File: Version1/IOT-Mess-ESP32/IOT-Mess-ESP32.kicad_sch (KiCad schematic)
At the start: 26 parts, among them J1 Conn_01x19_Pin, J10 Jumper, J2 Conn_01x19_Pin, J3 Jumper_2, J4 Jumper_2, J5 Conn_01x06_Pin, J7 Jumper, J8 Jumper, J9 Jumper, SW10 SW_Push, SW11 SW_Push, U10 USB_C_Receptacle_USB2.0_16P, U2 ESP32-C6-MINI-1, U4 ESP32-S2-WROVER, U6 ME6211C33M5

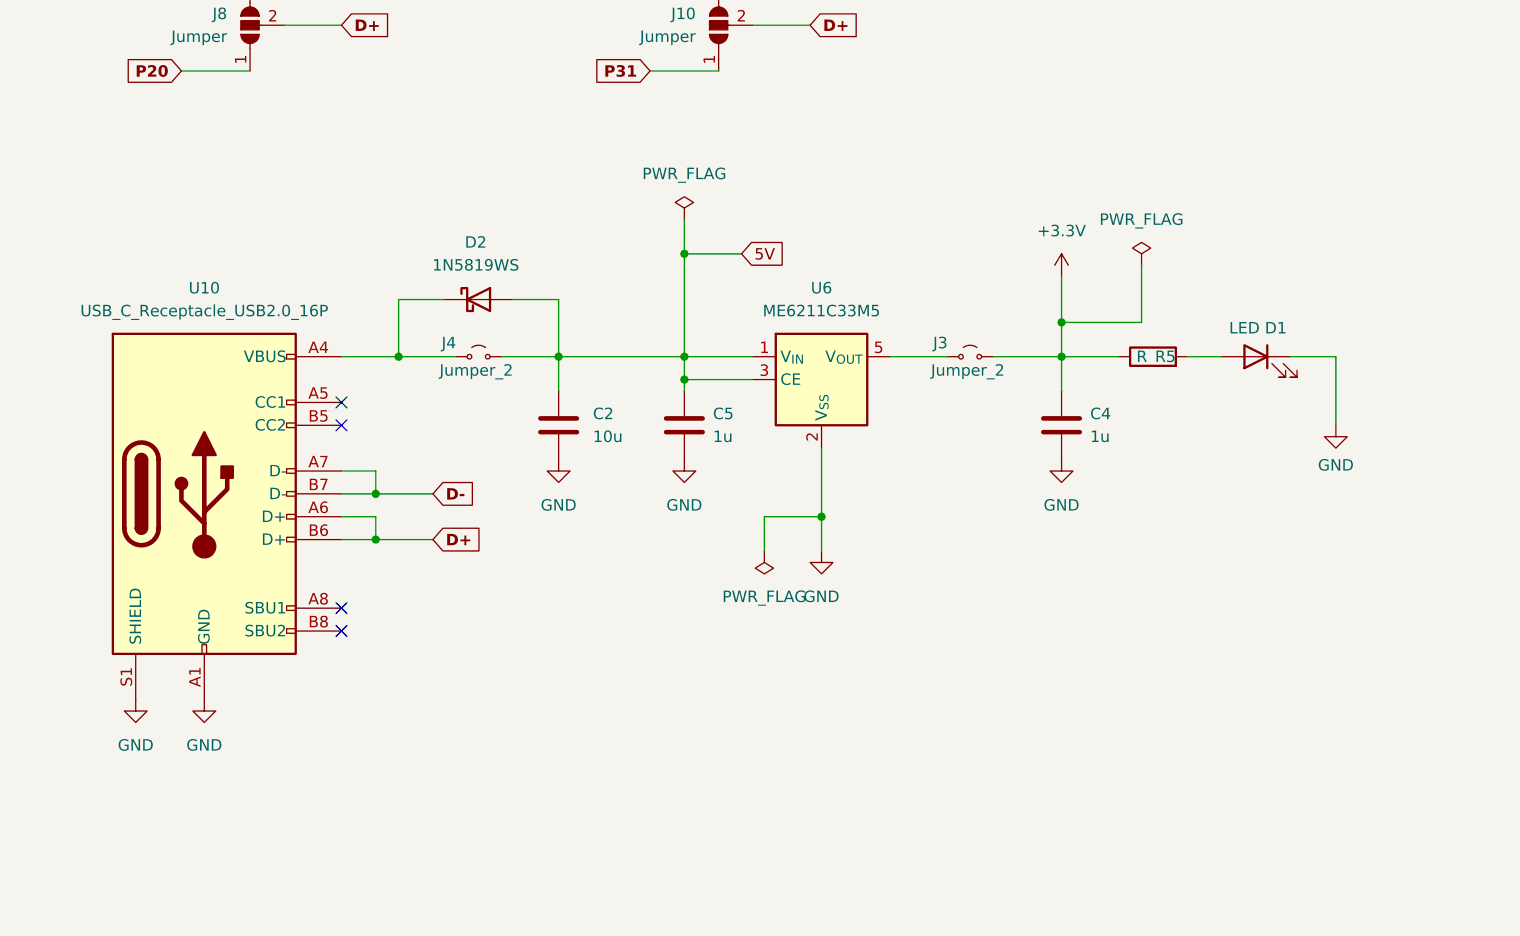
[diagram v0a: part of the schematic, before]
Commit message: updated.
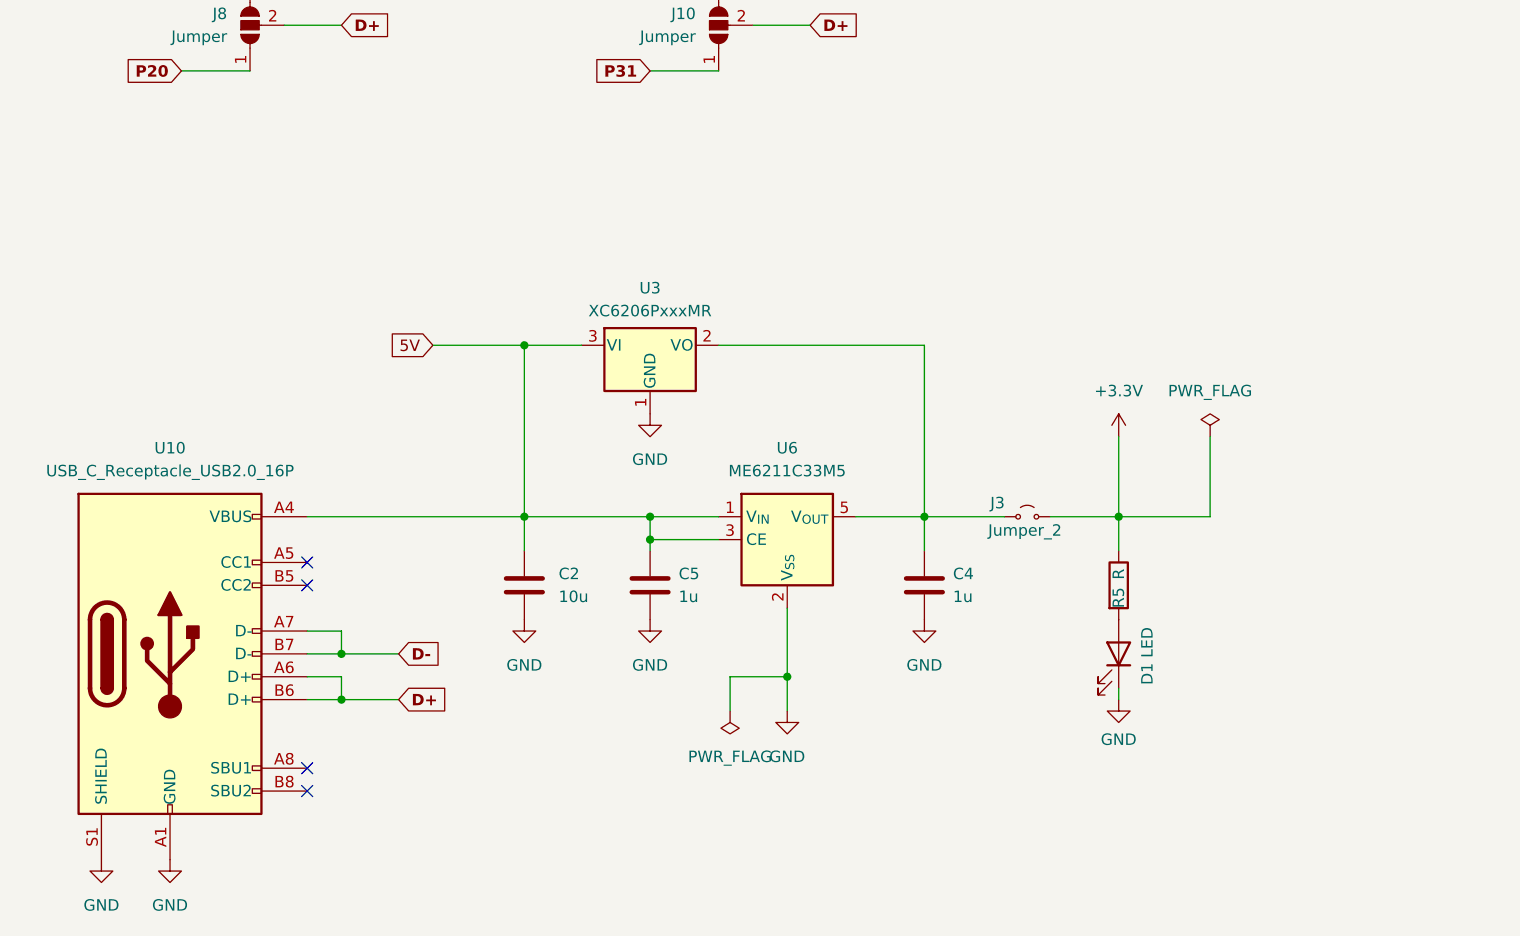
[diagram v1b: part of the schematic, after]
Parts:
- removed D2: 1N5819WS, Diode_SMD:D_SOD-323, symbol Diode:1N5819WS
- removed J4: Jumper_2, IOT-Mess-Footprints:Jumpper-triangle, symbol Jumper:Jumper_2_Small_Open
- added U3: XC6206PxxxMR, Package_TO_SOT_SMD:SOT-23-3, symbol Regulator_Linear:XC6206PxxxMR
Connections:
- net +3.3V: no longer C4.1
- net 5V: now also U10.A4 (VBUS), U10.A9 (VBUS), U10.B4 (VBUS), U10.B9 (VBUS), U3.3 (VI)
- net GND: now also U3.1 (GND)
- net at J3.1 (A), U6.5 (V_{OUT}): now also C4.1, U3.2 (VO)
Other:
- moved on the sheet: C2, C4, C5, D1, J3, R5, U10, U6
